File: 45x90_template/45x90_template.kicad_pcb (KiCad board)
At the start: 2 copper layers, 90 x 45 mm, 41 parts, among them J1 Screw_Terminal_01x02

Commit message: Edge vias 0.
Merge attempt.
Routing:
- net 0: vias 0 -> 170
- net (no net): vias 170 -> 0

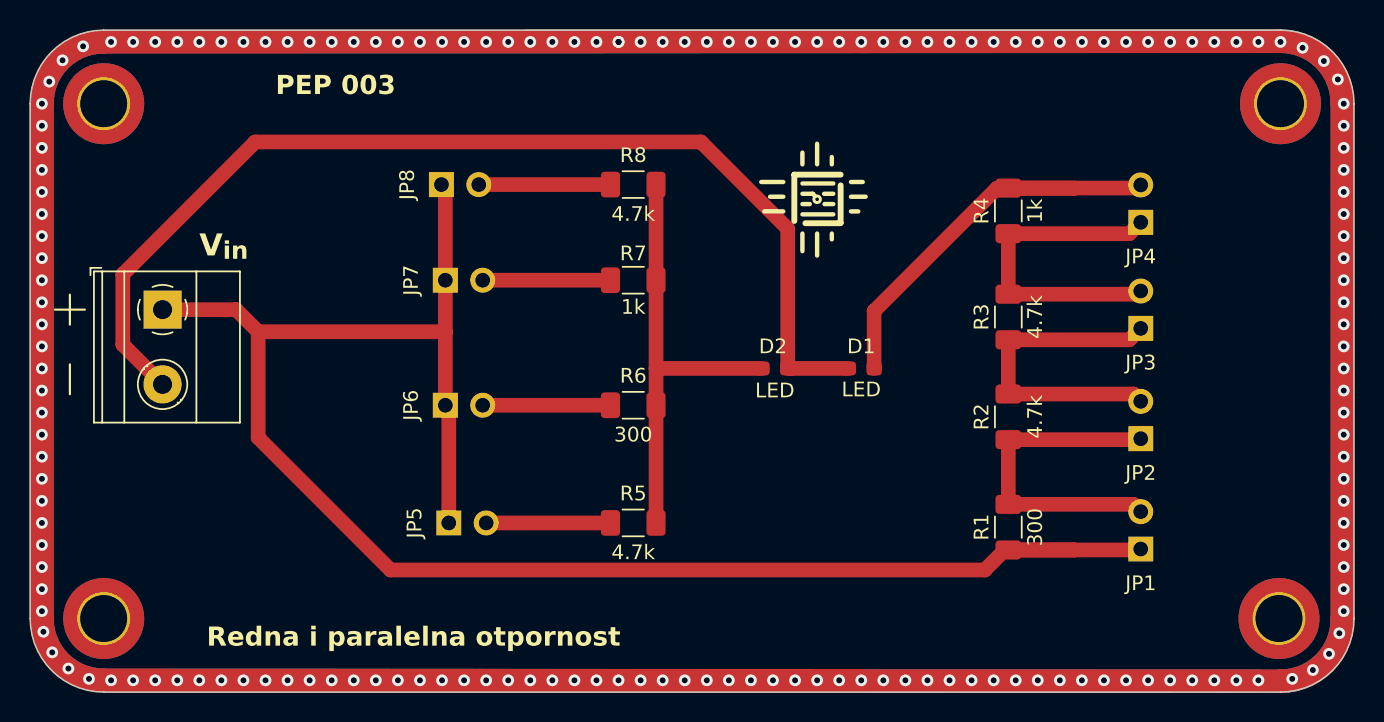
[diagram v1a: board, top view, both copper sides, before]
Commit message: Edge vias 0.
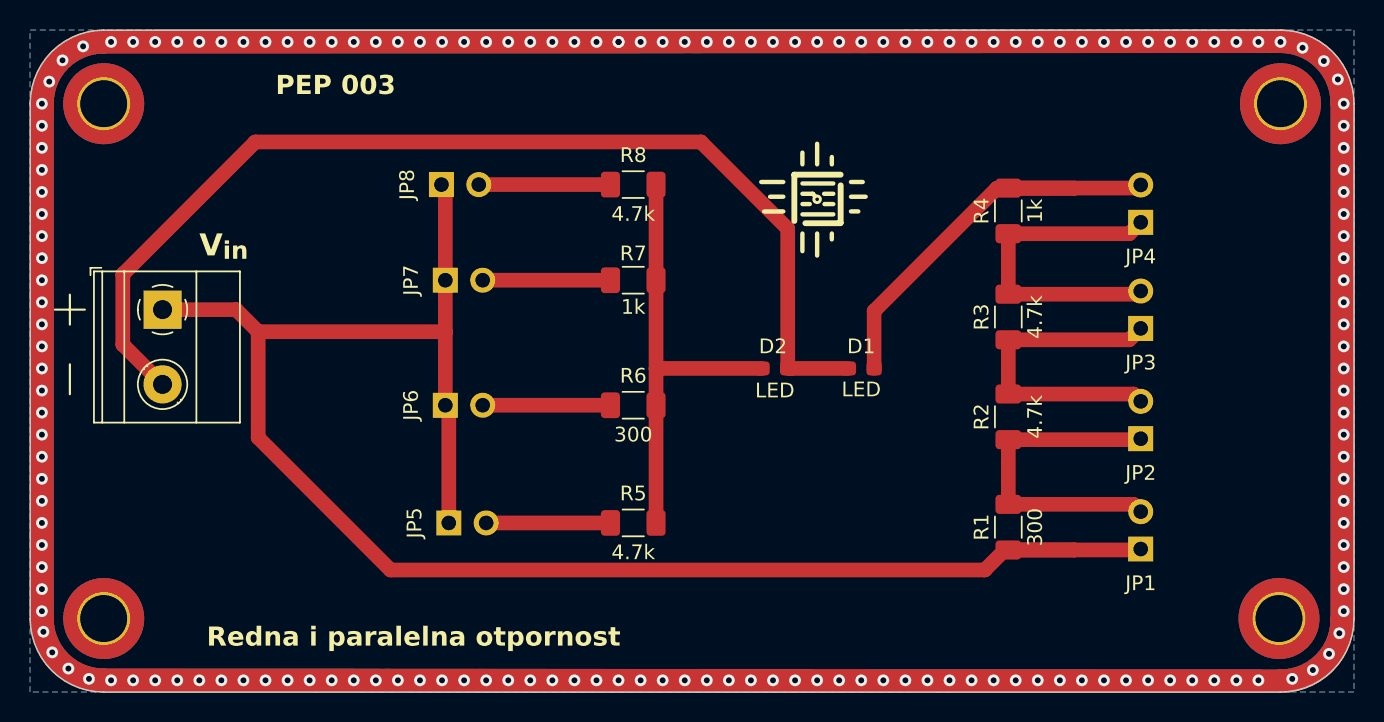
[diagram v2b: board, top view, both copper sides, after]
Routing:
- added copper zone on B.Cu, net 0
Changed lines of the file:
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@@
 		(net 11)
+	)
+	(zone
+		(net 1)
+		(net_name "0")
+		(layer "B.Cu")
+		(hatch edge 0.5)
+		(connect_pads
+			(clearance 0.5)
+		)
+		(min_thickness 0.25)
+		(filled_areas_thickness no)
+		(fill yes
+			(thermal_gap 0.5)
+			(thermal_bridge_width 0.5)
+		)
+		(polygon
+			(pts
+				(xy 100 105) (xy 190 105) (xy 190 150) (xy 100 150)
+			)
+		)
 	)
 	(embedded_fonts no)
